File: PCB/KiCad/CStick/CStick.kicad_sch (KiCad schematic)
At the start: 6 parts, among them J1 Conn_01x04_Male, U1 Stickbox_Assembly

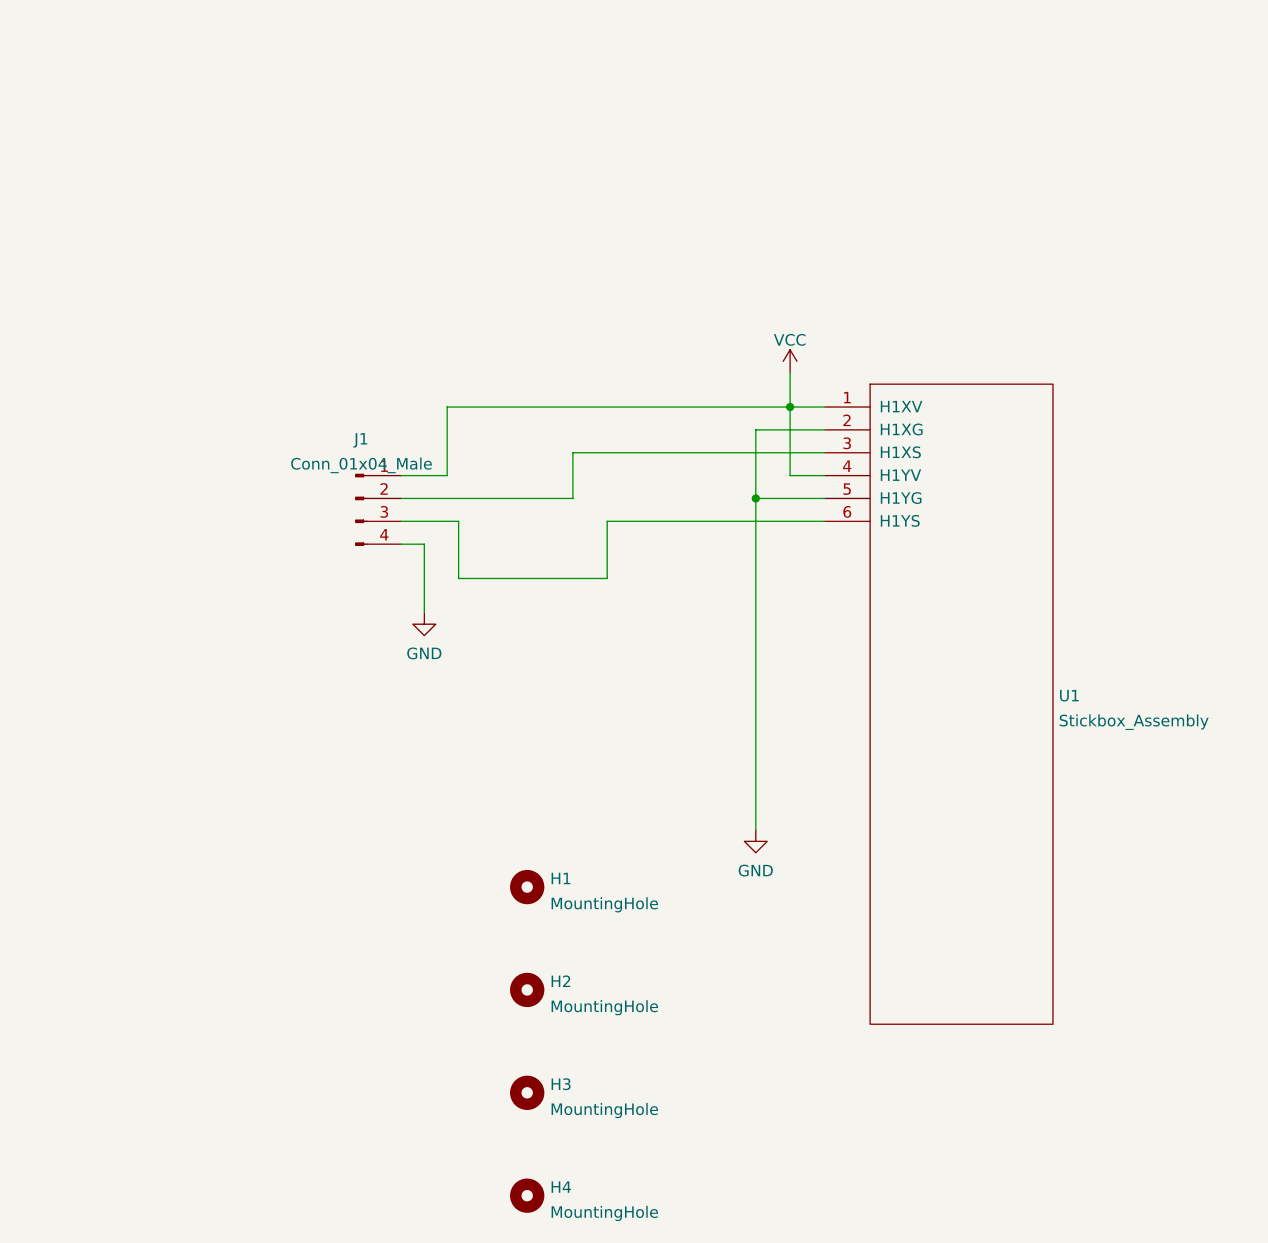
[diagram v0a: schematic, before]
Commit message: 1.2.2 overhaul
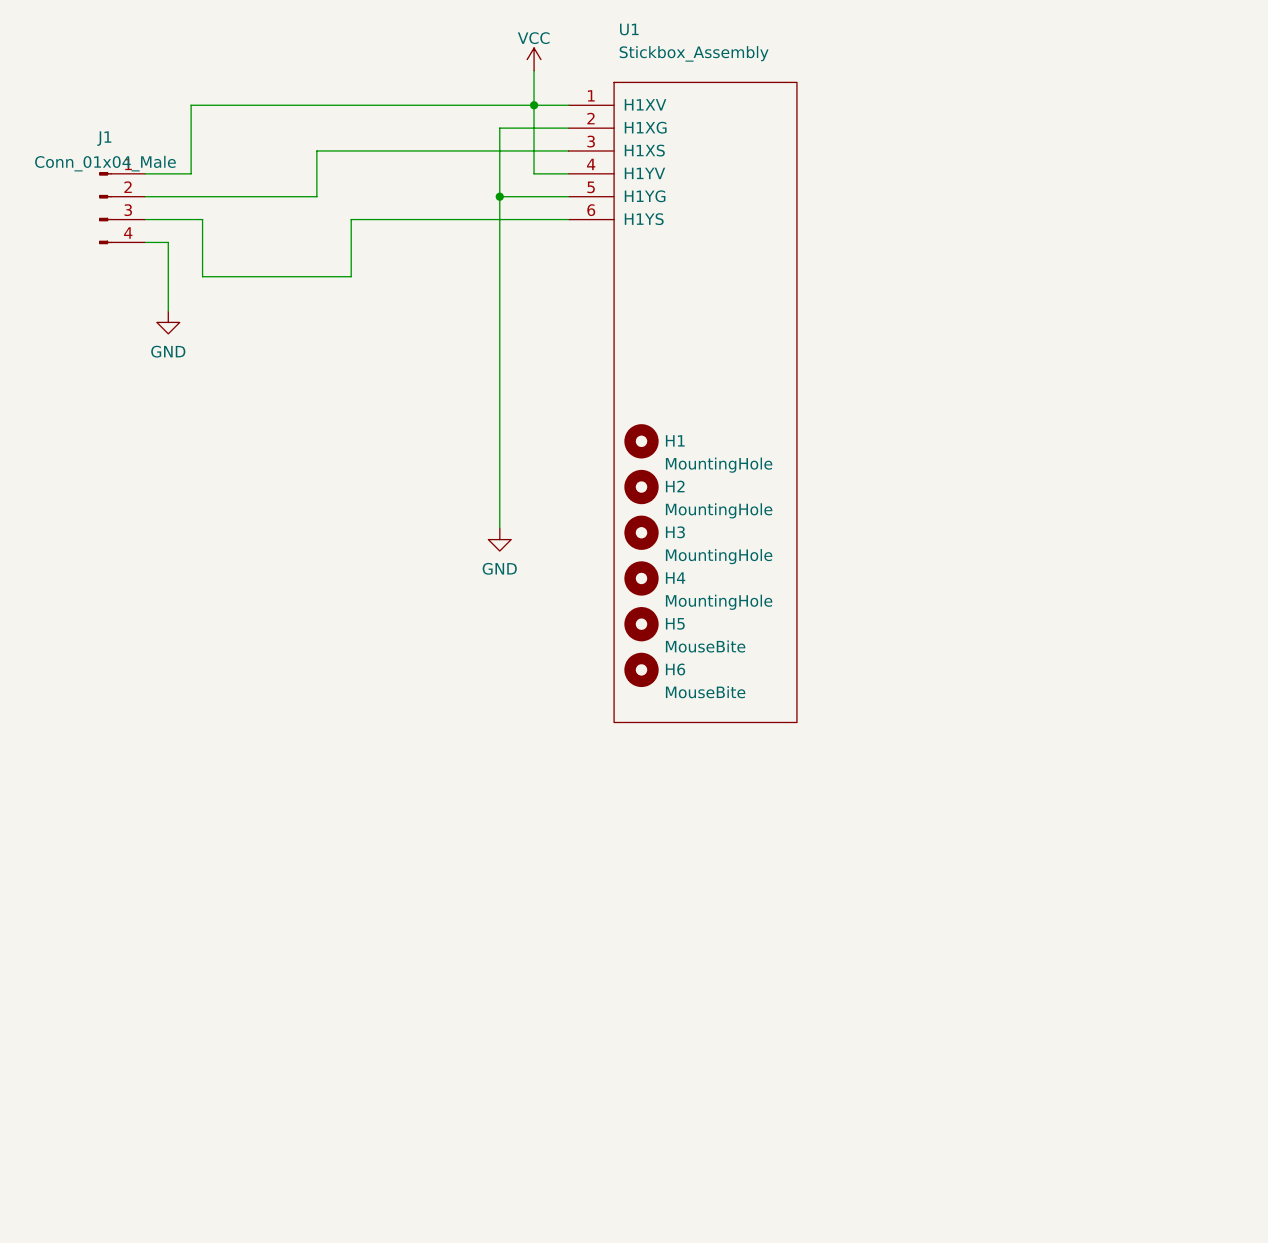
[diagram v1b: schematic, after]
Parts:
- added H5, H6: MouseBite, PhobGCC_Footprints:breakaway-mousebites-double, symbol Mechanical:MountingHole
- H1: footprint (none) -> PhobGCC_Footprints:MountingHole_1.8mm
- H2: footprint (none) -> PhobGCC_Footprints:MountingHole_5.2mm
- H3, H4: footprint (none) -> PhobGCC_Footprints:MountingHole_2.0mm
- U1: footprint (none) -> PhobGCC_Footprints:GCC_Stickbox_Hall_Only
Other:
- moved on the sheet: H1, H2, H3, H4, J1, U1
